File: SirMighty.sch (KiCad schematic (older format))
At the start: 40 parts, among them J1 Conn_01x20, J2 Conn_01x20, J3 USB_B_Micro, Q1 Q_DUAL_PMOS_S1G1D2S2G2D1, U1 ATmega1284P-MU, U2 AP7365-W-7, U3 FT231XQ, U4 AZ1117-5.0, Y1 20MHz

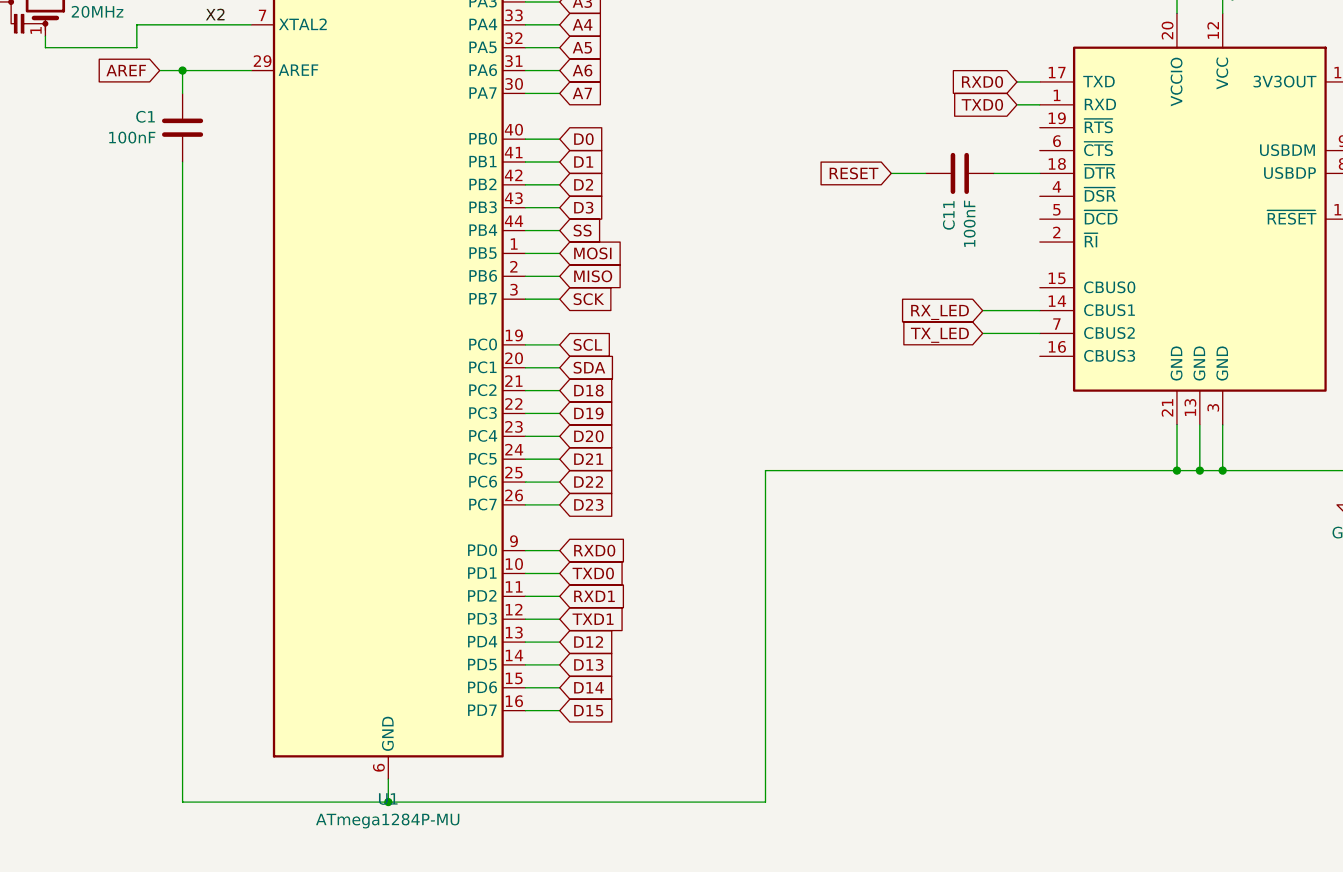
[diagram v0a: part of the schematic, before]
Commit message: Page Settings Updated
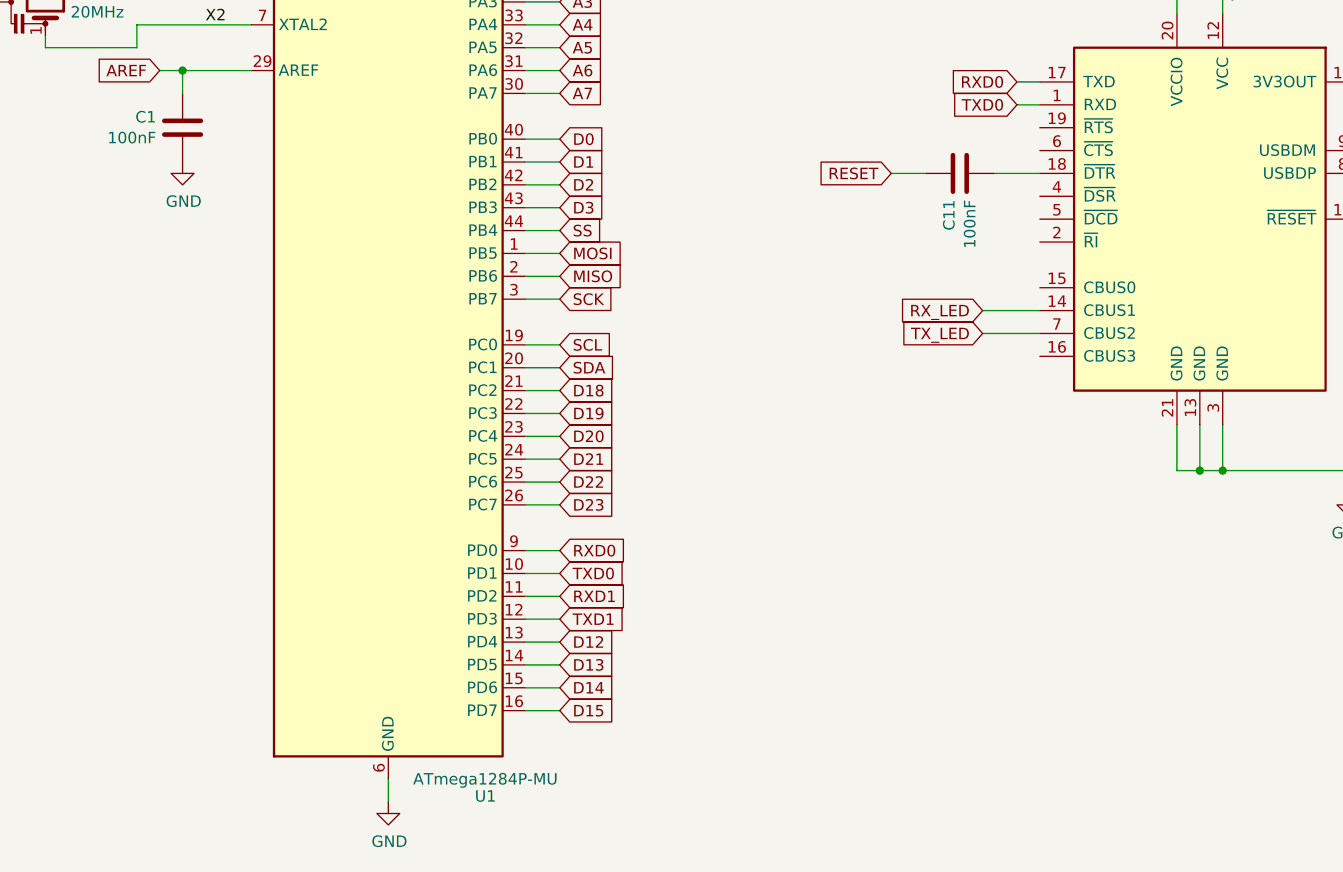
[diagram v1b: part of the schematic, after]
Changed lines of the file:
@@
 encoding utf-8
 Sheet 1 1
-Title ""
-Date ""
-Rev ""
-Comp ""
-Comment1 ""
-Comment2 ""
+Title "SirMighty"
+Date "2019-08-11"
+Rev "1"
+Comp "SirBoard"
+Comment1 "www.SirBoard.com"
+Comment2 "ATMega1284 Based Dev Board"
 Comment3 ""
 Comment4 ""
@@
 U 1 1 5D524CE7
 P 4350 5400
-F 0 "U1" H 4350 3312 50  0000 C CNN
-F 1 "ATmega1284P-MU" H 4350 3222 50  0000 C CNN
+F 0 "U1" H 4775 3325 50  0000 C CNN
+F 1 "ATmega1284P-MU" H 4775 3400 50  0000 C CNN
 F 2 "Package_DFN_QFN:QFN-44-1EP_7x7mm_P0.5mm_EP5.2x5.2mm" H 4350 5400 50  0001 C CIN
 F 3 "http://ww1.microchip.com/downloads/en/DeviceDoc/Atmel-8272-8-bit-AVR-microcontroller-ATmega164A_PA-324A_PA-644A_PA-1284_P_datasheet.pdf" H 4350 5400 50  0001 C CNN
@@
 Wire Wire Line
 	5100 6700 4950 6700
-Wire Wire Line
-	3450 4700 3450 7500
-Wire Wire Line
-	3450 7500 4350 7500
 Wire Wire Line
 	4350 7500 4350 7400
@@
 MISO
 Wire Wire Line
-	7800 6050 6000 6050
-Wire Wire Line
-	6000 6050 6000 7500
-Wire Wire Line
-	6000 7500 4350 7500
-Connection ~ 7800 6050
-Connection ~ 4350 7500
-Wire Wire Line
 	10700 2000 10850 2000
 Wire Wire Line
@@
 	1    0    0    -1
 $EndComp
+$Comp
+L power:GND #PWR?
+U 1 1 5DEF7311
+P 4350 7500
+F 0 "#PWR?" H 4350 7250 50  0001 C CNN
+F 1 "GND" H 4355 7327 50  0000 C CNN
+F 2 "" H 4350 7500 50  0001 C CNN
+F 3 "" H 4350 7500 50  0001 C CNN
+	1    4350 7500
+	1    0    0    -1
+$EndComp
+$Comp
+L power:GND #PWR?
+U 1 1 5DF0D40E
+P 3450 4700
+F 0 "#PWR?" H 3450 4450 50  0001 C CNN
+F 1 "GND" H 3455 4527 50  0000 C CNN
+F 2 "" H 3450 4700 50  0001 C CNN
+F 3 "" H 3450 4700 50  0001 C CNN
+	1    3450 4700
+	1    0    0    -1
+$EndComp
